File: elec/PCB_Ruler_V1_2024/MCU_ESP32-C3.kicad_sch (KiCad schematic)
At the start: 1 part, among them U2 ESP32-C3-WROOM-02-H4

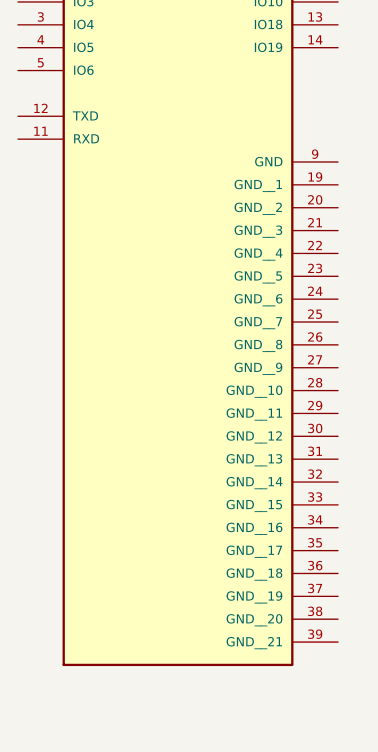
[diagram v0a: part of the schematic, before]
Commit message: IMU
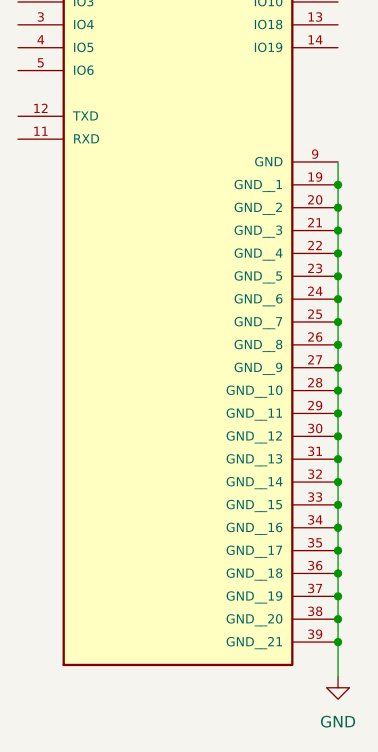
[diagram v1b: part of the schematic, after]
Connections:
- net GND: now reaches U2.19 (GND__1)
- net GND: now also U2.20 (GND__2), U2.21 (GND__3), U2.22 (GND__4), U2.23 (GND__5), U2.24 (GND__6), U2.25 (GND__7), U2.26 (GND__8), U2.27 (GND__9), U2.28 (GND__10), U2.29 (GND__11), U2.30 (GND__12), U2.31 (GND__13), U2.32 (GND__14), U2.33 (GND__15), U2.34 (GND__16), U2.35 (GND__17), U2.36 (GND__18), U2.37 (GND__19), U2.38 (GND__20), U2.39 (GND__21), U2.9 (GND)

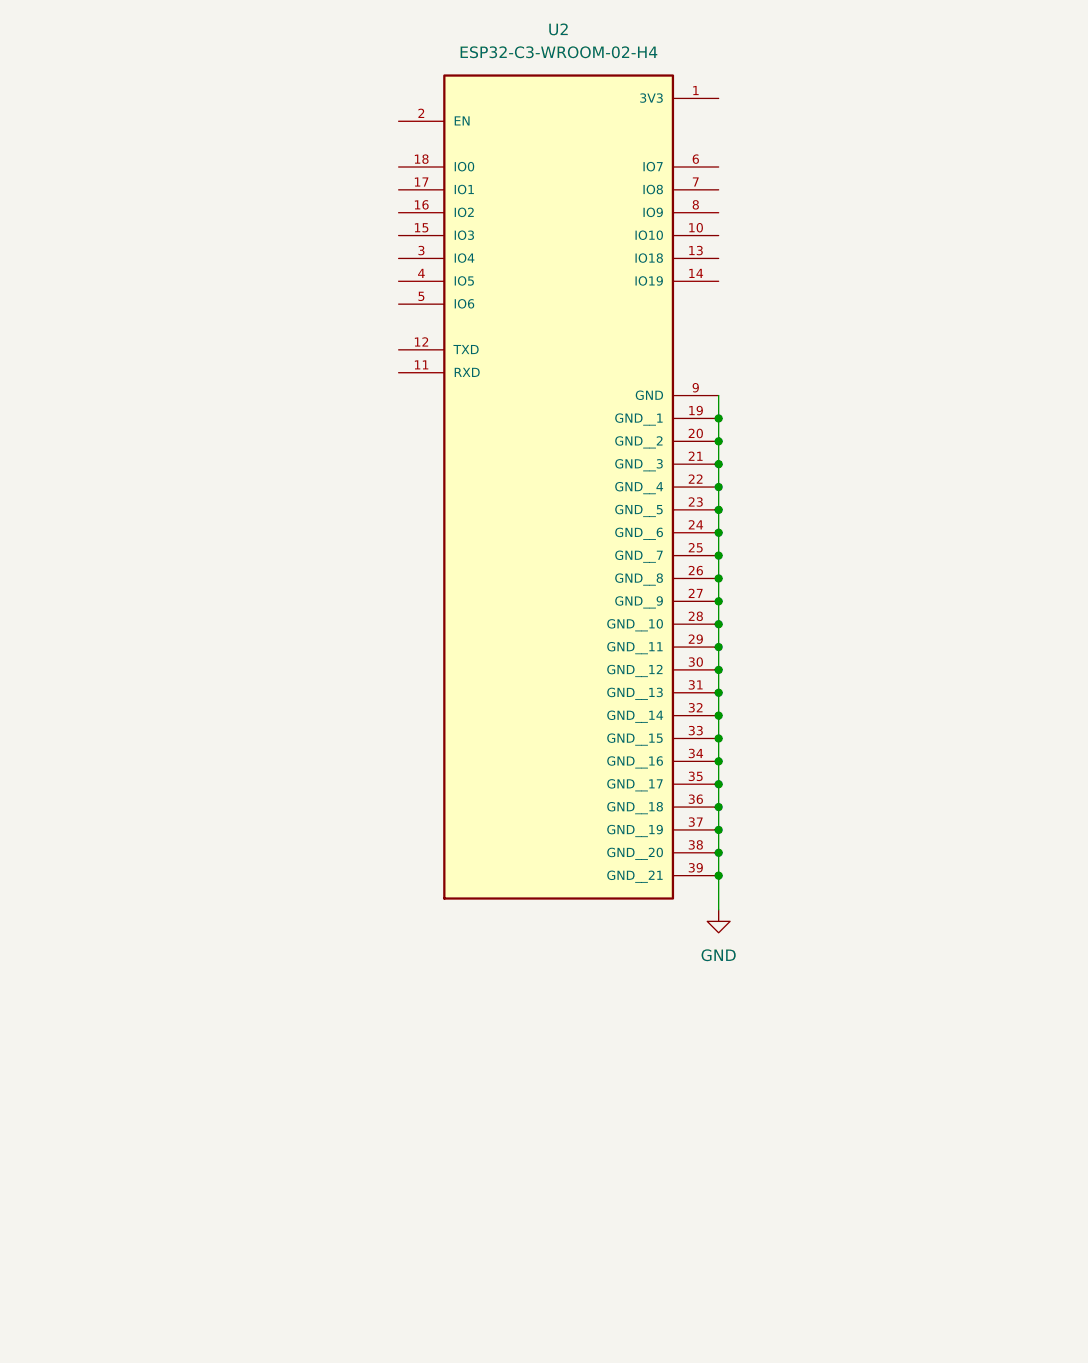
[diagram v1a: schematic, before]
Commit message: battery charger
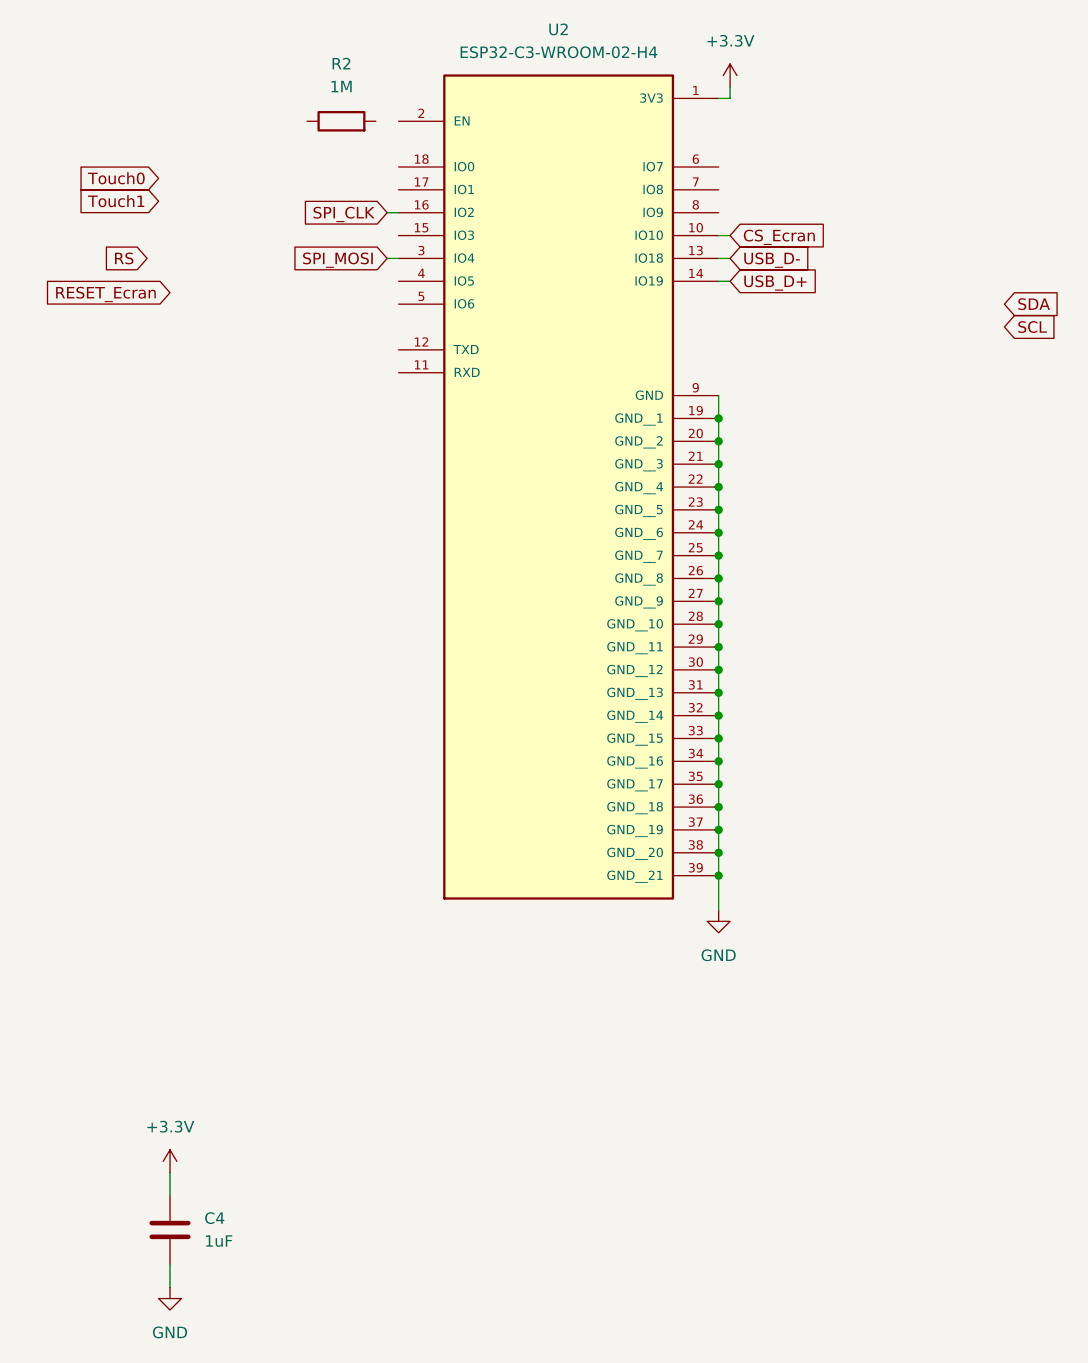
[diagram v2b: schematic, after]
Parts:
- added C4: 1uF, symbol Device:C
- added R2: 1M, symbol Device:R
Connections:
- net GND: now also C4.2
- net +3.3V: now reaches U2.1 (3V3)
- net +3.3V: now also C4.1
- net CS_Ecran: now reaches U2.10 (IO10)
- net USB_D-: now reaches U2.13 (IO18)
- net USB_D+: now reaches U2.14 (IO19)
- net SPI_CLK: now reaches U2.16 (IO2)
- net SPI_MOSI: now reaches U2.3 (IO4)

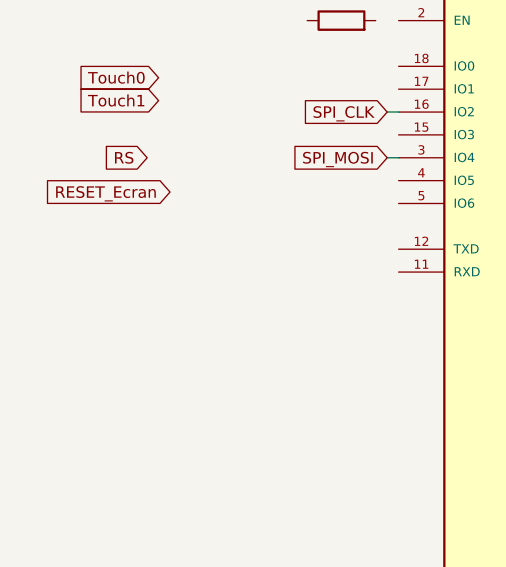
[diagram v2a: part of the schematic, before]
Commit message: Laser
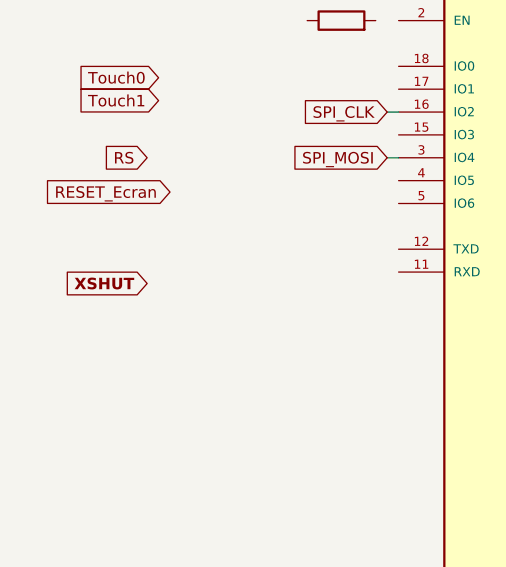
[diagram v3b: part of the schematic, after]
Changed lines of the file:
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@@
+		)
+	)
+	(global_label "XSHUT"
+		(shape input)
+		(at 34.29 81.28 180)
+		(fields_autoplaced yes)
+		(effects
+			(font
+				(size 1.27 1.27)
+				(thickness 0.254)
+				(bold yes)
+			)
+			(justify right)
+		)
+		(property "Intersheetrefs" "${INTERSHEET_REFS}"
+			(at 24.7812 81.28 0)
+			(effects
+				(font
+					(size 1.27 1.27)
+				)
+				(justify right)
+				(hide yes)
+			)
 		)
 	)
